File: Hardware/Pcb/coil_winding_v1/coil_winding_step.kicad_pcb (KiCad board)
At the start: 2 copper layers, 111.8 x 96.4 mm, 26 parts, among them J1 Conn_01x14_Pin, J2 Screw_Terminal_01x02, J3 Conn_01x03_Socket, J4 Conn_01x03_Socket, M1 Motor_DC, Q3 IRFZ40, SW1 SW_SPST, SW2 SW_SPST, SW3 RotaryEncoder_Switch, U1 LM7805_TO220

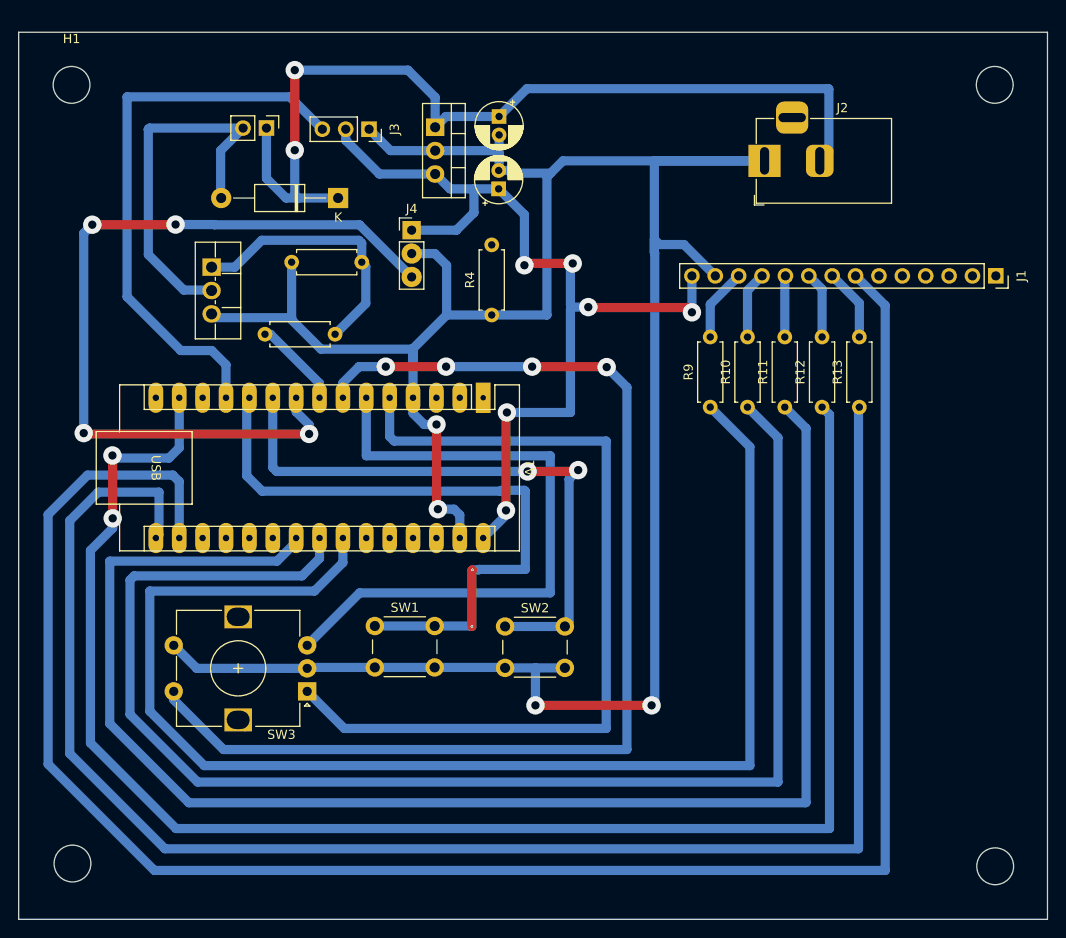
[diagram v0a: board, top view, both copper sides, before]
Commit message: tuesday
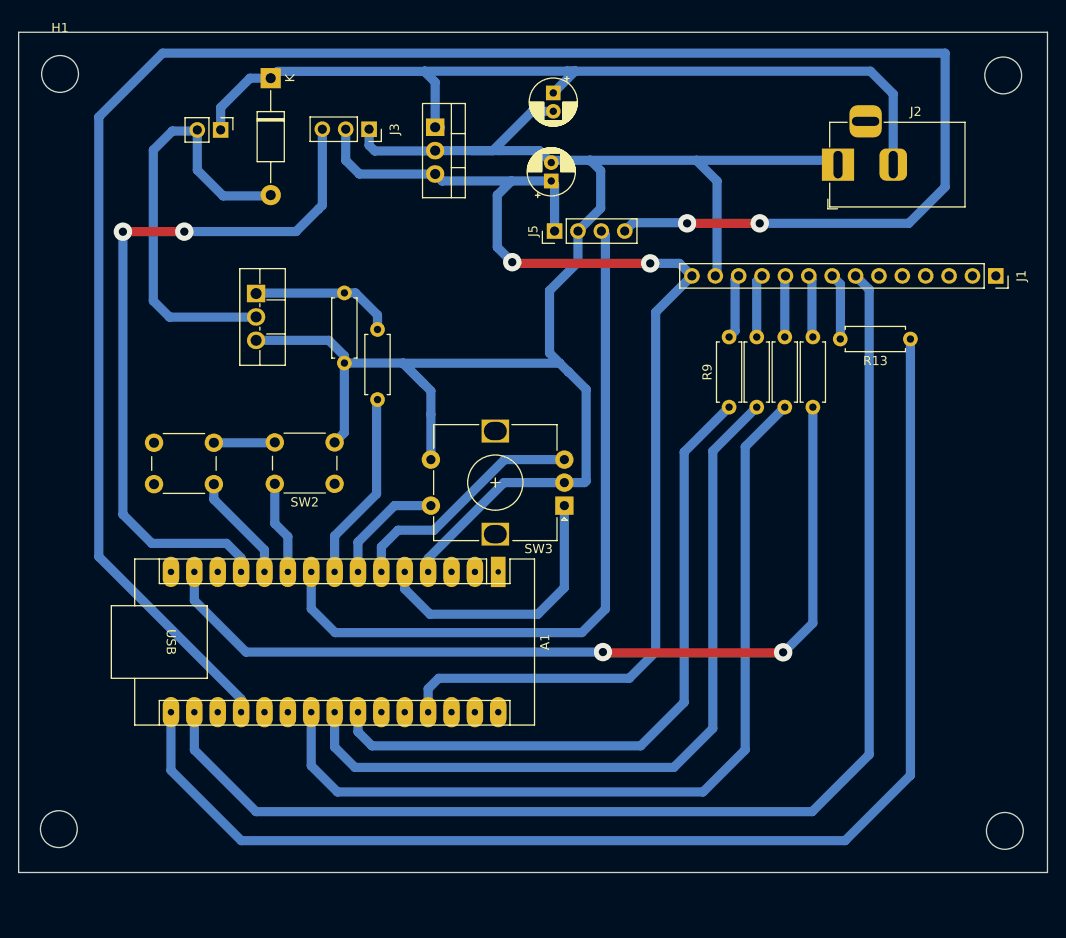
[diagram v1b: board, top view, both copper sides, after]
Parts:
- removed J4: Conn_01x03_Socket, Connector_PinHeader_2.54mm:PinHeader_1x03_P2.54mm_Vertical
- removed R4: R_US, Resistor_THT:R_Axial_DIN0207_L6.3mm_D2.5mm_P7.62mm_Horizontal
- added J5: Conn_01x04_Socket, Connector_PinHeader_2.54mm:PinHeader_1x04_P2.54mm_Vertical, F.Cu at (155.0, 72.7)
- moved SW3 34.5 mm to (156.1, 102.5)
- moved SW2 24.2 mm to (131.1, 100.1), turned to 180 degrees
- moved SW1 23.3 mm to (118.0, 100.2), turned to 180 degrees
- moved A1 19.0 mm to (148.9, 109.7)
- moved D1 14.9 mm to (124.2, 56.1), turned to -90 degrees
- moved R1 14.1 mm to (135.8, 91.0), turned to 90 degrees
- moved R2 12.4 mm to (132.2, 87.0), turned to 90 degrees
- moved R13 9.25 mm to (193.7, 84.4), turned to 180 degrees
- moved J2 7.99 mm to (185.8, 65.5)
- moved C1 6.42 mm to (154.9, 57.7)
- moved C2 5.78 mm to (154.7, 67.2)
- moved Q3 5.62 mm to (122.6, 79.5)
- moved M1 4.98 mm to (118.8, 61.7)
- moved H3 4.02 mm to (101.2, 137.7)
- moved H4 3.99 mm to (204.0, 137.8)
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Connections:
- A1 pad 19: unconnected-(A1-A0-Pad19) -> A0
- A1 pad 30: +5V -> unconnected-(A1-VIN-Pad30)
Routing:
- net A0: track 0.00 -> 217.3 mm, vias 0 -> 2
- net D4: track 126.9 -> 12.8 mm, vias 4 -> 0
- net GND: track 287.0 -> 204.8 mm, vias 4 -> 0
- net D11: track 175.8 -> 97.5 mm
- net 3V3: track 211.2 -> 135.4 mm
- net A5: track 147.2 -> 74.3 mm
- net A4: track 153.9 -> 84.4 mm
- net A3: track 162.3 -> 95.1 mm
- net D2: track 93.3 -> 30.4 mm
- net D8: track 70.7 -> 11.8 mm, vias 2 -> 0
- net D7: track 65.1 -> 10.2 mm, vias 2 -> 0
- net D3: track 70.0 -> 27.3 mm
- net D13: track 179.4 -> 140.2 mm
- net +5V: track 100.2 -> 133.9 mm, vias 6 -> 2
- net D9: track 61.8 -> 78.2 mm, vias 0 -> 2
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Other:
- board size 111.8 x 96.4 mm -> 111.8 x 91.3 mm
